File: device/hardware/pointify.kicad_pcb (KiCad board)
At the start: 2 copper layers, 24.5 x 22.6 mm, 16 parts, among them J1 USB_C, J2 SWIO, J3 PWM, U1 CH32X033F8P6

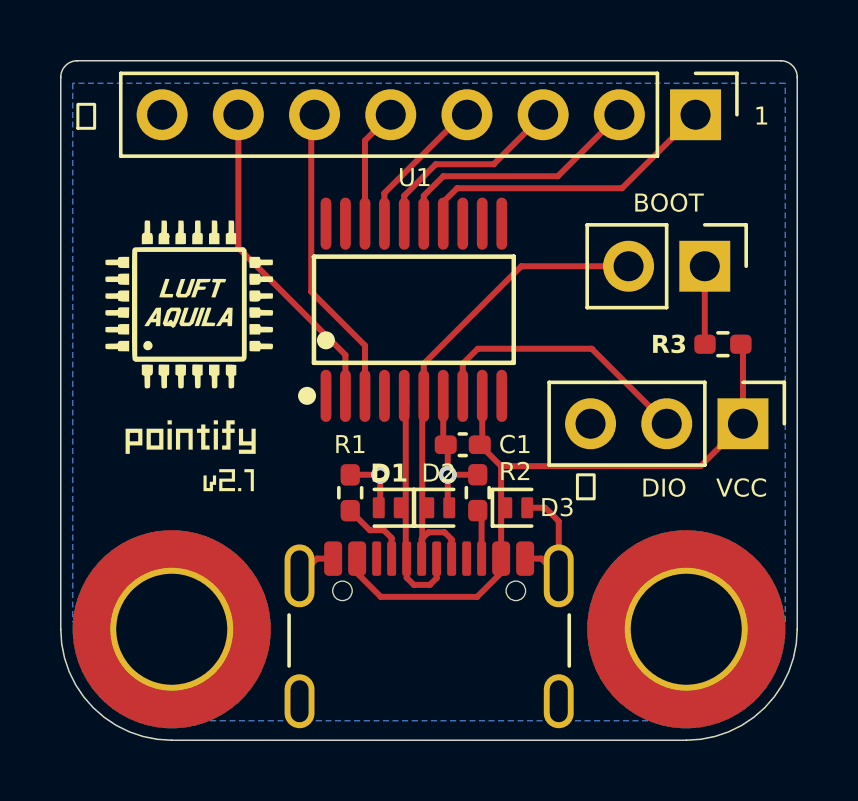
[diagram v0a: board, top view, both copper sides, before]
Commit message: update: pcb v2.2
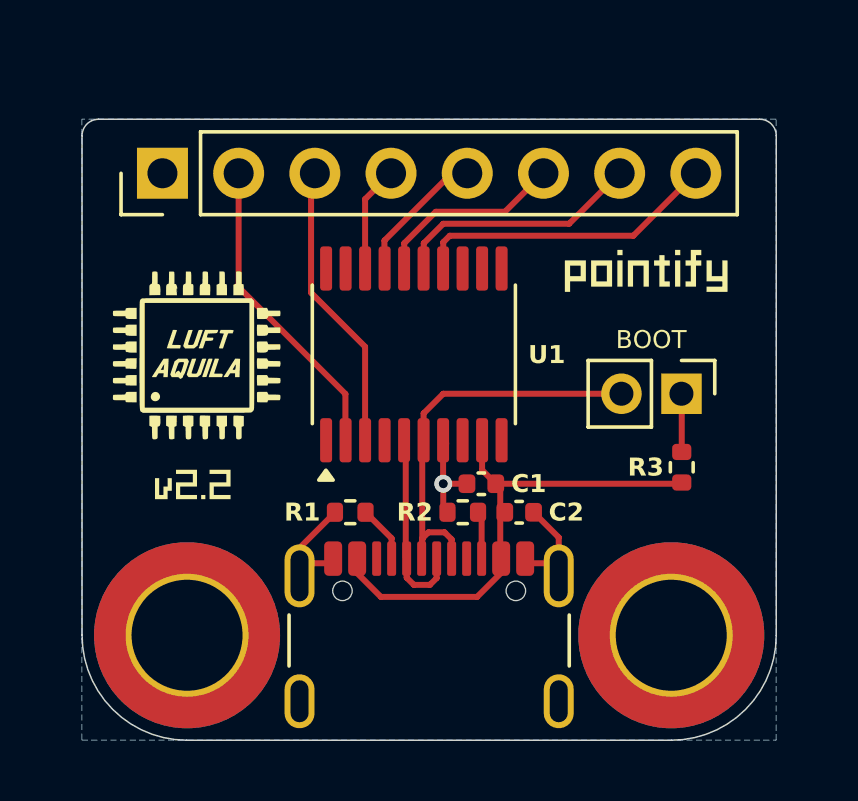
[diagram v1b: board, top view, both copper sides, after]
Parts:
- removed D1, D2, D3: H5VL10B, Diode_SMD:D_SOD-882
- removed the J2 at (163.9, 110.0)
- added C2: 1uF, Capacitor_SMD:C_0402_1005Metric, F.Cu at (156.4, 113.0)
- C1: footprint Capacitor_SMD:C_0402_1005Metric_Pad0.74x0.62mm_HandSolder -> Capacitor_SMD:C_0402_1005Metric
- JP1: footprint Connector_PinHeader_2.54mm:PinHeader_1x02_P2.54mm_Vertical -> Connector_PinHeader_2.00mm:PinHeader_1x02_P2.00mm_Vertical
- R1, R2, R3: footprint Resistor_SMD:R_0402_1005Metric_Pad0.72x0.64mm_HandSolder -> Resistor_SMD:R_0402_1005Metric
- U1: footprint ch32x033f8p6:CH32X033F8P6 -> Package_SO:TSSOP-20_4.4x6.5mm_P0.65mm
- moved J2 17.9 mm to (144.5, 101.7), turned to 90 degrees
- moved R3 4.32 mm to (161.8, 111.5), turned to 90 degrees
- moved JP1 4.32 mm to (161.8, 109.0)
- moved G*** 1.72 mm to (145.7, 107.7)
- moved U1 1.49 mm to (152.9, 107.7), turned to 90 degrees
- moved C1 1.44 mm to (155.2, 112.0)
- moved G*** 1.40 mm to (153.4, 108.5)
- moved R2 0.82 mm to (154.6, 113.0), turned to 180 degrees
- moved R1 0.65 mm to (150.8, 113.0), turned to 180 degrees
- moved H1 0.55 mm to (145.4, 117.0)
- moved H2 0.54 mm to (161.5, 117.0)
- renumbered J3 to J2
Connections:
- J2 pad 1: /PWM1_T2C1 -> GND
- J2 pad 2: /PWM2_T2C2 -> /PWM1_T1C1N
- J2 pad 3: /PWM3_T2C3 -> /PWM2_T1C3N
- J2 pad 4: /PWM4_T2C4 -> /PWM3_T3C1
- J2 pad 5: /PWM5_T3C1 -> /PWM4_T2C4
- J2 pad 6: /PWM6_T1C3N -> /PWM5_T2C3
- J2 pad 7: /PWM7_T1C1N -> /PWM6_T2C2
- J2 pad 8: GND -> /PWM7_T2C1
- U1 pad 14: /PWM1_T2C1 -> /PWM7_T2C1
- U1 pad 15: /PWM2_T2C2 -> /PWM6_T2C2
- U1 pad 16: /PWM3_T2C3 -> /PWM5_T2C3
- U1 pad 18: /PWM5_T3C1 -> /PWM3_T3C1
- U1 pad 2: /PWM7_T1C1N -> /PWM1_T1C1N
- U1 pad 3: /PWM6_T1C3N -> /PWM2_T1C3N
- U1 pad 8: /DIO -> unconnected-(U1-PC18/DIO-Pad8)
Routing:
- net /PWM7_T1C1N: track 10.8 -> 0.00 mm
- net /PWM1_T1C1N: track 0.00 -> 10.4 mm
- net /PWM7_T2C1: track 0.00 -> 10.3 mm
- net /PWM1_T2C1: track 10.3 -> 0.00 mm
- net /PWM6_T1C3N: track 10.2 -> 0.00 mm
- net /PWM2_T1C3N: track 0.00 -> 10.0 mm
- net /DIO: track 9.11 -> 0.00 mm
- net /PWM2_T2C2: track 8.57 -> 0.00 mm
- net /PWM6_T2C2: track 0.00 -> 8.43 mm
- net /PWM3_T2C3: track 6.68 -> 0.00 mm
- net /PWM5_T2C3: track 0.00 -> 6.54 mm
- net +5V: track 23.7 -> 17.2 mm
- net /PWM5_T3C1: track 3.99 -> 0.00 mm
- net /PWM3_T3C1: track 0.00 -> 3.53 mm
- net /UDP: track 17.3 -> 14.2 mm
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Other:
- board size 24.5 x 22.6 mm -> 23.1 x 20.7 mm
- board text added: "7"
- board text added: "https://github.com/luftaquila/pointify"
- board text removed: "1"
- board text removed: "DIO"
- board text removed: "VCC"
